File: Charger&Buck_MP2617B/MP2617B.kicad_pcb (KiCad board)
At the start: 2 copper layers, 50.2 x 17.5 mm, 43 parts, among them J1 Jumper

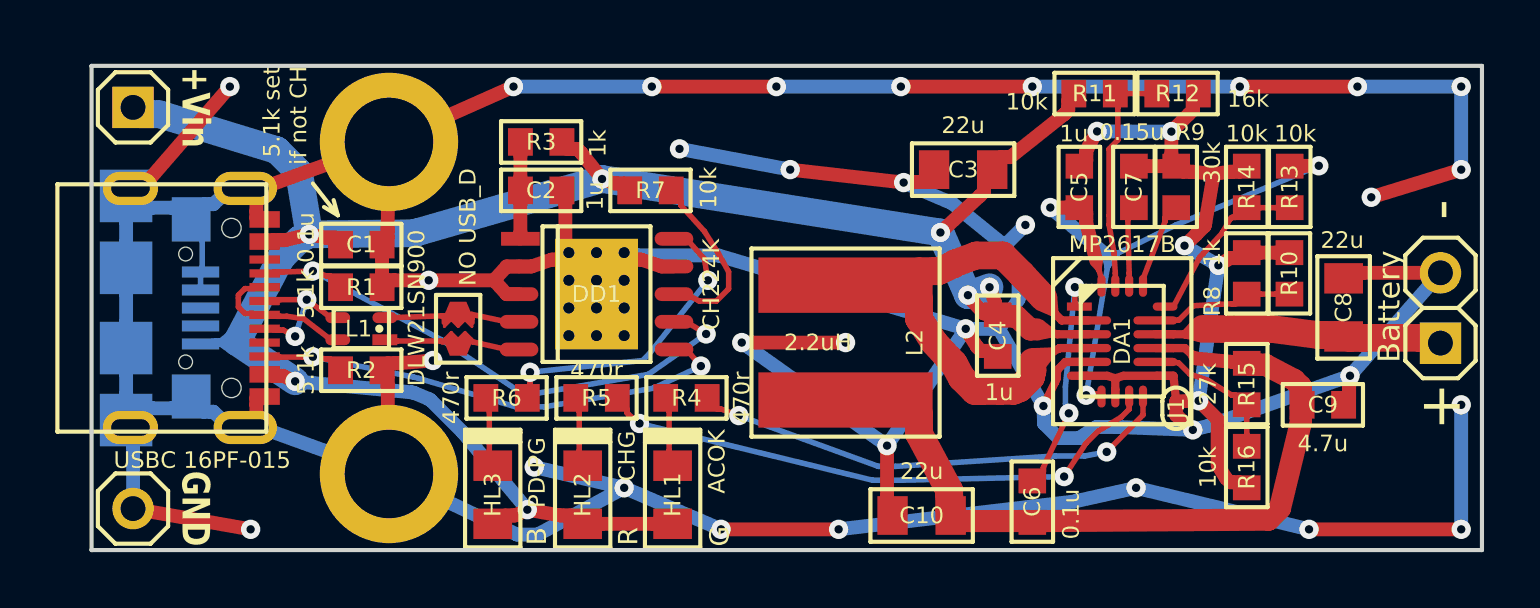
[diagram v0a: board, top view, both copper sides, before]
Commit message: исправления и дополнения
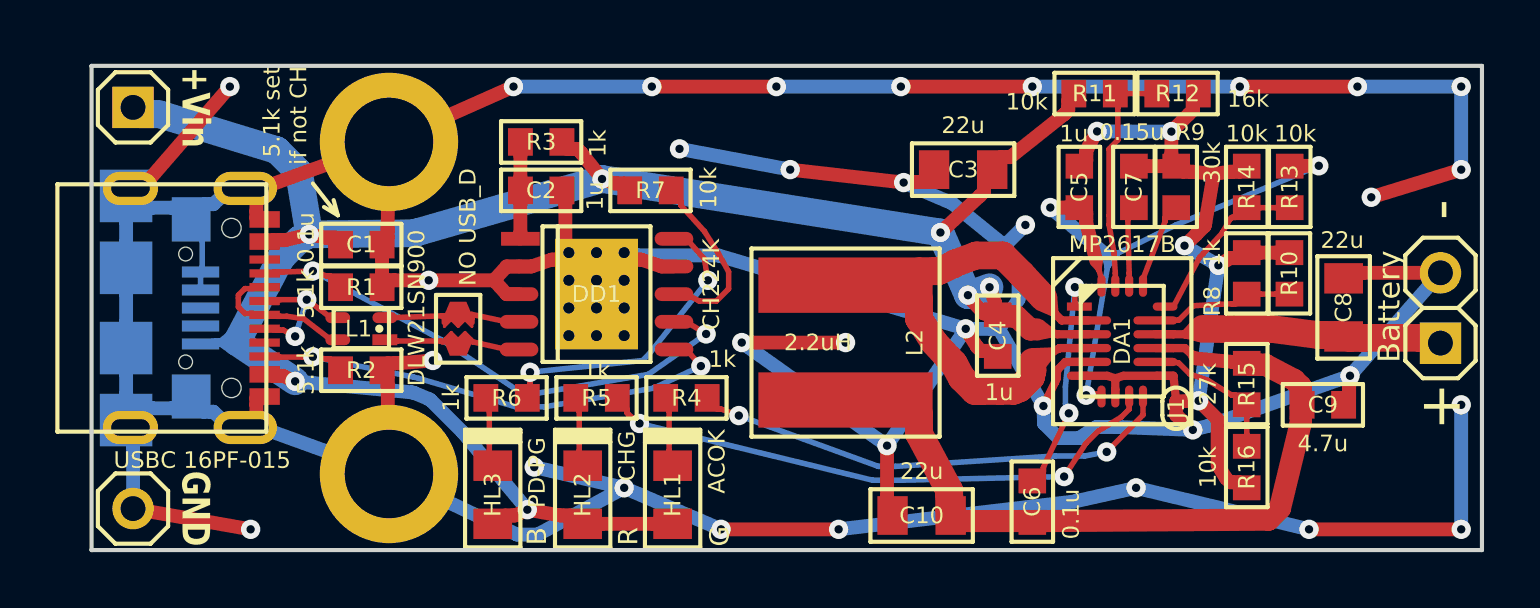
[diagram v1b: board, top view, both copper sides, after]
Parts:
- R4, R5, R6: value 470r -> 1k
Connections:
- C1 pad 2: GNDP -> GND
- C10 pad 2: GNDP -> GND
- C2 pad 2: GNDP -> GND
- C3 pad 2: GNDP -> GND
- C4 pad 2: GNDP -> GND
- C5 pad 1: /MP_VCC -> /+MP_VCC
- C5 pad 2: GND -> GNDL
- C7 pad 2: GND -> GNDL
- C8 pad 2: GNDP -> GND
- C9 pad 2: GNDP -> GND
- DA1 pad 11: GND -> GNDL
- DA1 pad 20: /MP_VCC -> /+MP_VCC
- DA1 pad 5: GNDP -> GND
- DA1 pad 6: GND -> GNDL
- DA1 pad 7: /MP_VCC -> /+MP_VCC
- DA1 pad 8: GND -> GNDL
- DD1 pad PAD: GNDP -> GND
- GB1 pad 2: GNDP -> GND
- Hole1 pad H: GNDP -> GND
- Hole2 pad H: GNDP -> GND
- J1 pad 1: GND -> GNDL
- J1 pad 2: GNDP -> GND
- R1 pad 2: GNDP -> GND
- R10 pad 2: GND -> GNDL
- R12 pad 2: GND -> GNDL
- R14 pad 2: GND -> GNDL
- R16 pad 2: GND -> GNDL
- R2 pad 2: GNDP -> GND
- R8 pad 2: GND -> GNDL
- R9 pad 2: GND -> GNDL
- XP2 pad 1: GNDP -> GND
- XS1 pad A1B12: GNDP -> GND
- XS1 pad B1A12: GNDP -> GND
- XS1 pad SHLD: GNDP -> GND
- XS2 pad 4: GNDP -> GND
- XS2 pad 5: GNDP -> GND
- XS2 pad SHLD: GNDP -> GND
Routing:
- net GNDL: track 0.00 -> 33.4 mm, vias 0 -> 5
- net GND: track 33.4 -> 0.00 mm, vias 5 -> 0
